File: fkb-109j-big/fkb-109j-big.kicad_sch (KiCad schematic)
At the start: 187 parts

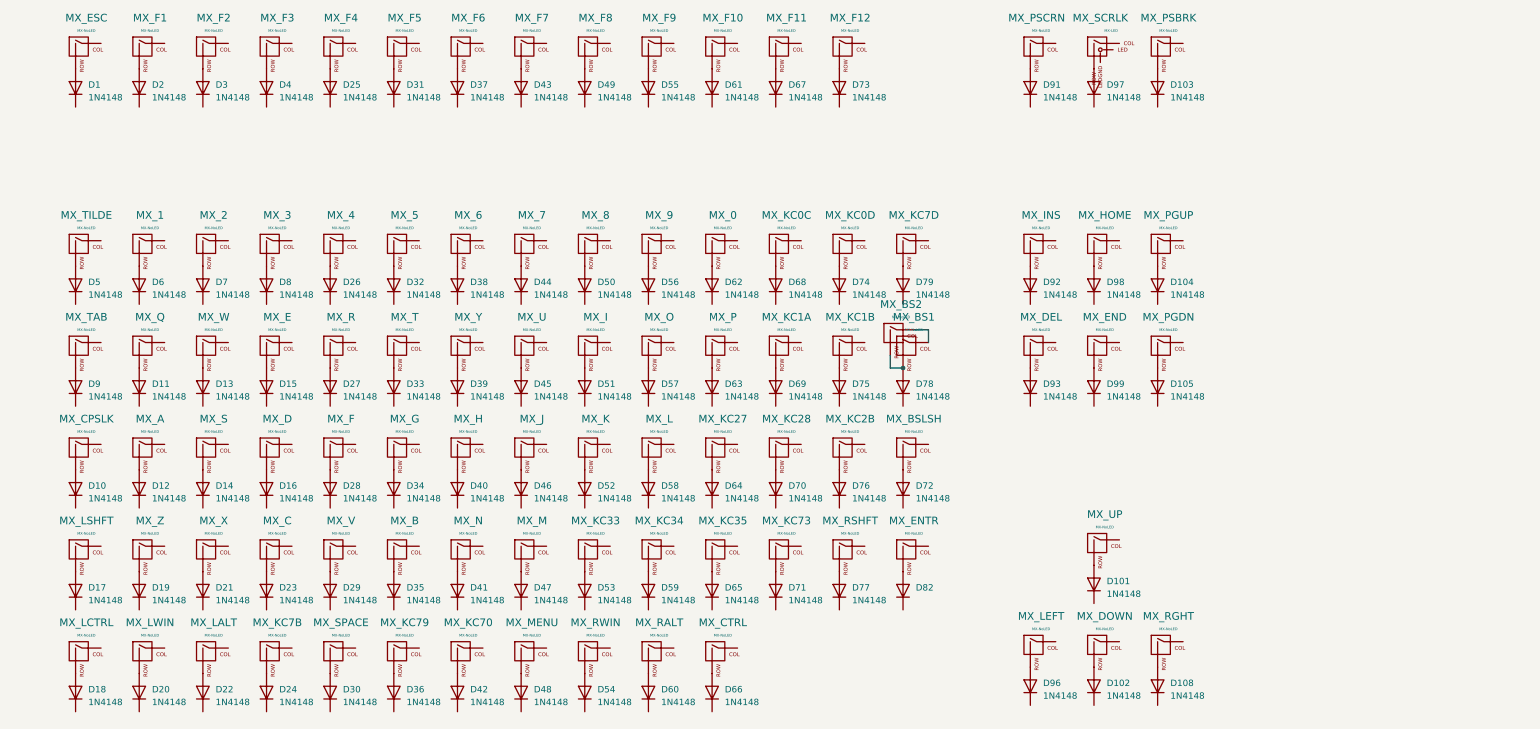
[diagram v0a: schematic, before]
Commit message: start board layout
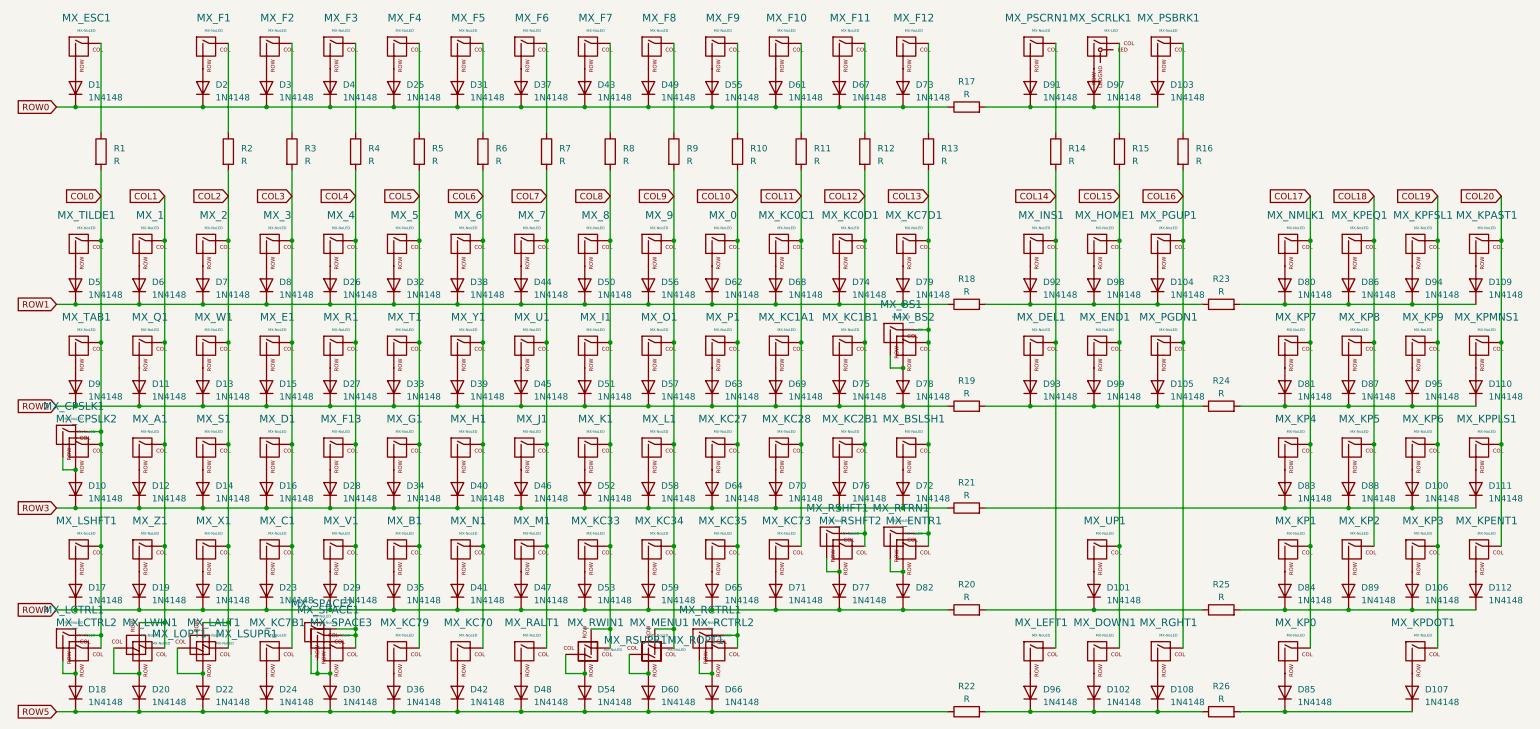
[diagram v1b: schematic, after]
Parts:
- added D100, D106, D107, D109, D110, D111, D112, D80, D81, D83, D84, D85, D86, D87, D88, D89, D94, D95: 1N4148, Diode_THT:D_DO-35_SOD27_P7.62mm_Horizontal, symbol Diode:1N4148
- added MX_CPSLK1, MX_LSUPR1, MX_RSUPR1: MX-NoLED, Alps_Only:ALPS-1.5U, symbol MX_Alps_Hybrid:MX-NoLED
- added MX_KP0, MX_KP1, MX_KP2, MX_KP3, MX_KP4, MX_KP5, MX_KP6, MX_KP7, MX_KP8, MX_KP9, MX_KPAST1, MX_KPDOT1, MX_KPEQ1, MX_KPFSL1, MX_KPMNS1, MX_KPPLS1, MX_NMLK1: MX-NoLED, Alps_Only:ALPS-1U, symbol MX_Alps_Hybrid:MX-NoLED
- added MX_KPENT1: MX-NoLED, Alps_Only:ALPS-2U, symbol MX_Alps_Hybrid:MX-NoLED
- added MX_LCTRL1, MX_LOPT1, MX_RCTRL1, MX_ROPT1: MX-NoLED, Alps_Only:ALPS-1.25U, symbol MX_Alps_Hybrid:MX-NoLED
- added MX_RSHFT1: MX-NoLED, Alps_Only:ALPS-2.75U, symbol MX_Alps_Hybrid:MX-NoLED
- added MX_RTRN1: MX-NoLED, Alps_Only:ALPS-2.25U, symbol MX_Alps_Hybrid:MX-NoLED
- added MX_SPACE1: MX-NoLED, Alps_Only:ALPS-6.5U, symbol MX_Alps_Hybrid:MX-NoLED
- added MX_SPACE2: MX-NoLED, Alps_Only:ALPS-6.25U, symbol MX_Alps_Hybrid:MX-NoLED
- added R1, R10, R11, R12, R13, R14, R15, R16, R17, R18, R19, R2, R20, R21, R22, R23, R24, R25, R26, R3, R4, R5, R6, R7, R8, R9: R, Resistor_THT:R_Axial_DIN0207_L6.3mm_D2.5mm_P10.16mm_Horizontal, symbol Device:R
- MX_0, MX_1, MX_2, MX_3, MX_4, MX_5, MX_6, MX_7, MX_8, MX_9, MX_F1, MX_F10, MX_F11, MX_F12, MX_F2, MX_F3, MX_F4, MX_F5, MX_F6, MX_F7, MX_F8, MX_F9, MX_KC27, MX_KC28, MX_KC33, MX_KC34, MX_KC35, MX_KC73: footprint (none) -> Alps_Only:ALPS-1U
- MX_A1: renamed from MX_A; footprint (none) -> Alps_Only:ALPS-1U
- MX_B1: renamed from MX_B; footprint (none) -> Alps_Only:ALPS-1U
- MX_BS2: renamed from MX_BS1; footprint Alps_Only:ALPS-1U -> Alps_Only:ALPS-2U
- MX_BSLSH1: renamed from MX_BSLSH; footprint (none) -> Alps_Only:ALPS-1.5U
- MX_C1: renamed from MX_C; footprint (none) -> Alps_Only:ALPS-1U
- MX_CPSLK2: renamed from MX_CPSLK; footprint (none) -> Alps_Only:ALPS-1.75U
- MX_D1: renamed from MX_D; footprint (none) -> Alps_Only:ALPS-1U
- MX_DEL1: renamed from MX_DEL; footprint (none) -> Alps_Only:ALPS-1U
- MX_DOWN1: renamed from MX_DOWN; footprint (none) -> Alps_Only:ALPS-1U
- MX_E1: renamed from MX_E; footprint (none) -> Alps_Only:ALPS-1U
- MX_END1: renamed from MX_END; footprint (none) -> Alps_Only:ALPS-1U
- MX_ENTR1: renamed from MX_ENTR; footprint (none) -> Alps_Only:ALPS-2U
- MX_ESC1: renamed from MX_ESC; footprint (none) -> Alps_Only:ALPS-1U
- MX_F13: renamed from MX_F; footprint (none) -> Alps_Only:ALPS-1U
- MX_G1: renamed from MX_G; footprint (none) -> Alps_Only:ALPS-1U
- MX_H1: renamed from MX_H; footprint (none) -> Alps_Only:ALPS-1U
- MX_HOME1: renamed from MX_HOME; footprint (none) -> Alps_Only:ALPS-1U
- MX_I1: renamed from MX_I; footprint (none) -> Alps_Only:ALPS-1U
- MX_INS1: renamed from MX_INS; footprint (none) -> Alps_Only:ALPS-1U
- MX_J1: renamed from MX_J; footprint (none) -> Alps_Only:ALPS-1U
- MX_K1: renamed from MX_K; footprint (none) -> Alps_Only:ALPS-1U
- MX_KC0C1: renamed from MX_KC0C; footprint (none) -> Alps_Only:ALPS-1U
- MX_KC0D1: renamed from MX_KC0D; footprint (none) -> Alps_Only:ALPS-1U
- MX_KC1A1: renamed from MX_KC1A; footprint (none) -> Alps_Only:ALPS-1U
- MX_KC1B1: renamed from MX_KC1B; footprint (none) -> Alps_Only:ALPS-1U
- MX_KC2B1: renamed from MX_KC2B; footprint (none) -> Alps_Only:ALPS-1U
- MX_KC70, MX_KC79: footprint (none) -> Alps_Only:ALPS-1.25U
- MX_KC7B1: renamed from MX_KC7B; footprint (none) -> Alps_Only:ALPS-1.25U
- MX_KC7D1: renamed from MX_KC7D; footprint (none) -> Alps_Only:ALPS-1U
- MX_L1: renamed from MX_L; footprint (none) -> Alps_Only:ALPS-1U
- MX_LALT1: renamed from MX_LALT; footprint (none) -> Alps_Only:ALPS-1.25U
- MX_LCTRL2: renamed from MX_LCTRL; footprint (none) -> Alps_Only:ALPS-1.5U
- MX_LEFT1: renamed from MX_LEFT; footprint (none) -> Alps_Only:ALPS-1U
- MX_LSHFT1: renamed from MX_LSHFT; footprint (none) -> Alps_Only:ALPS-2.25U
- MX_LWIN1: renamed from MX_LWIN; footprint (none) -> Alps_Only:ALPS-1.25U
- MX_M1: renamed from MX_M; footprint (none) -> Alps_Only:ALPS-1U
- MX_MENU1: renamed from MX_MENU; footprint (none) -> Alps_Only:ALPS-1.25U
- MX_N1: renamed from MX_N; footprint (none) -> Alps_Only:ALPS-1U
- MX_O1: renamed from MX_O; footprint (none) -> Alps_Only:ALPS-1U
- MX_P1: renamed from MX_P; footprint (none) -> Alps_Only:ALPS-1U
- MX_PGDN1: renamed from MX_PGDN; footprint (none) -> Alps_Only:ALPS-1U
- MX_PGUP1: renamed from MX_PGUP; footprint (none) -> Alps_Only:ALPS-1U
- MX_PSBRK1: renamed from MX_PSBRK; footprint (none) -> Alps_Only:ALPS-1U
- MX_PSCRN1: renamed from MX_PSCRN; footprint (none) -> Alps_Only:ALPS-1U
- MX_Q1: renamed from MX_Q; footprint (none) -> Alps_Only:ALPS-1U
- MX_R1: renamed from MX_R; footprint (none) -> Alps_Only:ALPS-1U
- MX_RALT1: renamed from MX_RALT; footprint (none) -> Alps_Only:ALPS-1.25U
- MX_RCTRL2: renamed from MX_CTRL; footprint (none) -> Alps_Only:ALPS-1.5U
- MX_RGHT1: renamed from MX_RGHT; footprint (none) -> Alps_Only:ALPS-1U
- MX_RSHFT2: renamed from MX_RSHFT; footprint (none) -> Alps_Only:ALPS-1.75U
- MX_RWIN1: renamed from MX_RWIN; footprint (none) -> Alps_Only:ALPS-1.25U
- MX_S1: renamed from MX_S; footprint (none) -> Alps_Only:ALPS-1U
- MX_SCRLK1: renamed from MX_SCRLK; footprint (none) -> Alps_Only:ALPS-1U
- MX_SPACE3: renamed from MX_SPACE; footprint (none) -> Alps_Only:ALPS-2.5U
- MX_T1: renamed from MX_T; footprint (none) -> Alps_Only:ALPS-1U
- MX_TAB1: renamed from MX_TAB; footprint (none) -> Alps_Only:ALPS-1.5U
- MX_TILDE1: renamed from MX_TILDE; footprint (none) -> Alps_Only:ALPS-1U
- MX_U1: renamed from MX_U; footprint (none) -> Alps_Only:ALPS-1U
- MX_UP1: renamed from MX_UP; footprint (none) -> Alps_Only:ALPS-1U
- MX_V1: renamed from MX_V; footprint (none) -> Alps_Only:ALPS-1U
- MX_W1: renamed from MX_W; footprint (none) -> Alps_Only:ALPS-1U
- MX_X1: renamed from MX_X; footprint (none) -> Alps_Only:ALPS-1U
- MX_Y1: renamed from MX_Y; footprint (none) -> Alps_Only:ALPS-1U
- MX_Z1: renamed from MX_Z; footprint (none) -> Alps_Only:ALPS-1U
- renumbered MX_BS2 to MX_BS1
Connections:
- net COL2: now reaches MX_S1.1 (COL)
- net COL2: now also MX_2.1 (COL), MX_LALT1.1 (COL), MX_W1.1 (COL), MX_X1.1 (COL), MX_LSUPR1.2 (ROW), R2.2
- net at D97.1 (K): now also D103.1 (K), D91.1 (K), R17.2
- net ROW4: now reaches D53.1 (K)
- net ROW4: now also D17.1 (K), D19.1 (K), D21.1 (K), D23.1 (K), D29.1 (K), D35.1 (K), D41.1 (K), D47.1 (K), D59.1 (K), D65.1 (K), D71.1 (K), D77.1 (K), D82.1 (K), R20.1
- net COL9: now reaches MX_O1.1 (COL)
- net COL9: now also MX_9.1 (COL), MX_KC34.1 (COL), MX_L1.1 (COL), MX_MENU1.1 (COL), MX_ROPT1.2 (ROW), R9.2
- net ROW5: now reaches D24.1 (K)
- net ROW5: now also D18.1 (K), D20.1 (K), D22.1 (K), D30.1 (K), D36.1 (K), D42.1 (K), D48.1 (K), D54.1 (K), D60.1 (K), D66.1 (K), R22.1
- net ROW3: now reaches D34.1 (K)
- net ROW3: now also D10.1 (K), D12.1 (K), D14.1 (K), D16.1 (K), D28.1 (K), D40.1 (K), D46.1 (K), D52.1 (K), D58.1 (K), D64.1 (K), D70.1 (K), D72.1 (K), D76.1 (K), R21.1
- net COL13: now reaches MX_BS1.1 (COL), MX_BS2.1 (COL)
- net COL13: now also MX_BSLSH1.1 (COL), MX_ENTR1.1 (COL), MX_KC7D1.1 (COL), MX_RTRN1.1 (COL), R13.2
- net ROW1: now reaches D68.1 (K)
- net ROW1: now also D26.1 (K), D32.1 (K), D38.1 (K), D44.1 (K), D5.1 (K), D50.1 (K), D56.1 (K), D6.1 (K), D62.1 (K), D7.1 (K), D74.1 (K), D79.1 (K), D8.1 (K), R18.1
- net COL10: now reaches MX_P1.1 (COL)
- net COL10: now also MX_0.1 (COL), MX_KC27.1 (COL), MX_KC35.1 (COL), MX_RCTRL2.1 (COL), MX_RCTRL1.1 (COL), R10.2
- net ROW0: now reaches D3.1 (K)
- net ROW0: now also D1.1 (K), D2.1 (K), D25.1 (K), D31.1 (K), D37.1 (K), D4.1 (K), D43.1 (K), D49.1 (K), D55.1 (K), D61.1 (K), D67.1 (K), D73.1 (K), R17.1
- net COL11: now reaches MX_KC73.1 (COL)
- net COL11: now also MX_KC0C1.1 (COL), MX_KC1A1.1 (COL), MX_KC28.1 (COL), R11.2
- net at MX_F6.1 (COL): now also R7.1
- net ROW2: now reaches D13.1 (K)
- net ROW2: now also D11.1 (K), D15.1 (K), D27.1 (K), D33.1 (K), D39.1 (K), D45.1 (K), D51.1 (K), D57.1 (K), D63.1 (K), D69.1 (K), D75.1 (K), D78.1 (K), D9.1 (K), R19.1
- net COL7: now reaches MX_U1.1 (COL)
- net COL7: now also MX_7.1 (COL), MX_J1.1 (COL), MX_M1.1 (COL), MX_RALT1.1 (COL), R7.2
- net at D96.1 (K): now also D102.1 (K), D108.1 (K), R22.2, R26.1
- net COL4: now reaches MX_V1.1 (COL)
- net COL4: now also MX_4.1 (COL), MX_F13.1 (COL), MX_R1.1 (COL), MX_SPACE3.1 (COL), MX_SPACE1.1 (COL), MX_SPACE2.1 (COL), R4.2
- net at D20.2 (A), MX_LWIN1.2 (ROW): now also MX_LOPT1.1 (COL)
- net COL1: now reaches MX_LWIN1.1 (COL)
- net COL1: now also MX_1.1 (COL), MX_A1.1 (COL), MX_Q1.1 (COL), MX_Z1.1 (COL), MX_LOPT1.2 (ROW)
- net COL6: now reaches MX_H1.1 (COL)
- net COL6: now also MX_6.1 (COL), MX_KC70.1 (COL), MX_N1.1 (COL), MX_Y1.1 (COL), R6.2
- net at D30.2 (A), MX_SPACE3.2 (ROW): now also MX_SPACE1.2 (ROW), MX_SPACE2.2 (ROW)
- net COL0: now reaches MX_TAB1.1 (COL)
- net COL0: now also MX_CPSLK2.1 (COL), MX_LCTRL2.1 (COL), MX_LSHFT1.1 (COL), MX_TILDE1.1 (COL), MX_CPSLK1.1 (COL), MX_LCTRL1.1 (COL), R1.2
- net at D93.1 (K): now also D105.1 (K), D99.1 (K), R19.2, R24.1
- net COL8: now reaches MX_I1.1 (COL)
- net COL8: now also MX_8.1 (COL), MX_K1.1 (COL), MX_KC33.1 (COL), MX_RWIN1.1 (COL), MX_RSUPR1.2 (ROW), R8.2
- net at D82.2 (A), MX_ENTR1.2 (ROW): now also MX_RTRN1.2 (ROW)
- net COL5: now reaches MX_5.1 (COL)
- net COL5: now also MX_B1.1 (COL), MX_G1.1 (COL), MX_KC79.1 (COL), MX_T1.1 (COL), R5.2
- net COL12: now reaches MX_KC0D1.1 (COL)
- net COL12: now also MX_KC1B1.1 (COL), MX_KC2B1.1 (COL), MX_RSHFT2.1 (COL), MX_RSHFT1.1 (COL), R12.2
- net at MX_MENU1.2 (ROW): now also D60.2 (A), MX_ROPT1.1 (COL); no longer D48.2 (A)
- net at D77.2 (A), MX_RSHFT2.2 (ROW): now also MX_RSHFT1.2 (ROW)
- net at D22.2 (A), MX_LALT1.2 (ROW): now also MX_LSUPR1.1 (COL)
- net at MX_PSCRN1.1 (COL): now also R14.1
- net at D54.2 (A), MX_RWIN1.2 (ROW): now also MX_RSUPR1.1 (COL)
- net at MX_F12.1 (COL): now also R13.1
- net at MX_F5.1 (COL): now also R6.1
- net COL14: now reaches MX_DEL1.1 (COL)
- net COL14: now also MX_INS1.1 (COL), MX_LEFT1.1 (COL), R14.2
- net at MX_F10.1 (COL): now also R11.1
- net at D98.1 (K): now also D104.1 (K), D92.1 (K), R18.2, R23.1
- net at MX_F4.1 (COL): now also R5.1
- net at D18.2 (A), MX_LCTRL2.2 (ROW): now also MX_LCTRL1.2 (ROW)
- net at MX_F8.1 (COL): now also R9.1
- net at MX_ESC1.1 (COL): now also R1.1
- net at MX_F7.1 (COL): now also R8.1
- net COL16: now reaches MX_PGDN1.1 (COL)
- net COL16: now also MX_PGUP1.1 (COL), MX_RGHT1.1 (COL), R16.2
- net at D66.2 (A), MX_RCTRL2.2 (ROW): now also MX_RCTRL1.2 (ROW)
- net at MX_F9.1 (COL): now also R10.1
- net at MX_RALT1.2 (ROW): now also D48.2 (A); no longer D60.2 (A)
- net COL15: now reaches MX_HOME1.1 (COL)
- net COL15: now also MX_DOWN1.1 (COL), MX_END1.1 (COL), MX_UP1.1 (COL), R15.2
- net at D101.1 (K): now also R20.2, R25.1
- net at MX_SCRLK1.1 (COL): now also R15.1
- net COL3: now reaches MX_KC7B1.1 (COL)
- net COL3: now also MX_3.1 (COL), MX_C1.1 (COL), MX_D1.1 (COL), MX_E1.1 (COL), R3.2
- net at MX_F1.1 (COL): now also R2.1
- net at MX_F3.1 (COL): now also R4.1
- net at MX_F11.1 (COL): now also R12.1
- net at D10.2 (A), MX_CPSLK2.2 (ROW): now also MX_CPSLK1.2 (ROW)
- net at MX_F2.1 (COL): now also R3.1
- net at MX_PSBRK1.1 (COL): now also R16.1
- new net: D100.1 (K), D111.1 (K), D83.1 (K), D88.1 (K), R21.2
- new net: D106.1 (K), D112.1 (K), D84.1 (K), D89.1 (K), R25.2
- new net: D84.2 (A), MX_KP1.2 (ROW)
- new net: D81.2 (A), MX_KP7.2 (ROW)
- new net: D109.1 (K), D80.1 (K), D86.1 (K), D94.1 (K), R23.2
- new net: D89.2 (A), MX_KP2.2 (ROW)
- new net: D107.2 (A), MX_KPDOT1.2 (ROW)
- new net: D80.2 (A), MX_NMLK1.2 (ROW)
- new net: D107.1 (K), D85.1 (K), R26.2
- new net: D85.2 (A), MX_KP0.2 (ROW)
- new net: D110.1 (K), D81.1 (K), D87.1 (K), D95.1 (K), R24.2
- new net: D110.2 (A), MX_KPMNS1.2 (ROW)
- new net: D112.2 (A), MX_KPENT1.2 (ROW)
- new net: D86.2 (A), MX_KPEQ1.2 (ROW)
- new net: D88.2 (A), MX_KP5.2 (ROW)
- new net: D111.2 (A), MX_KPPLS1.2 (ROW)
- new net: D83.2 (A), MX_KP4.2 (ROW)
- new net: D95.2 (A), MX_KP9.2 (ROW)
- new net: D100.2 (A), MX_KP6.2 (ROW)
- new net: D94.2 (A), MX_KPFSL1.2 (ROW)
- new net: D87.2 (A), MX_KP8.2 (ROW)
- new net: D109.2 (A), MX_KPAST1.2 (ROW)
- new net: D106.2 (A), MX_KP3.2 (ROW)
- new net COL17: MX_KP0.1 (COL), MX_KP1.1 (COL), MX_KP4.1 (COL), MX_KP7.1 (COL), MX_NMLK1.1 (COL)
- new net COL18: MX_KP2.1 (COL), MX_KP5.1 (COL), MX_KP8.1 (COL), MX_KPEQ1.1 (COL)
- new net COL19: MX_KP3.1 (COL), MX_KP6.1 (COL), MX_KP9.1 (COL), MX_KPDOT1.1 (COL), MX_KPFSL1.1 (COL)
- new net COL20: MX_KPAST1.1 (COL), MX_KPENT1.1 (COL), MX_KPMNS1.1 (COL), MX_KPPLS1.1 (COL)
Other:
- moved on the sheet: D101, D102, D108, D2, D25, D3, D31, D37, D4, D43, D49, D55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

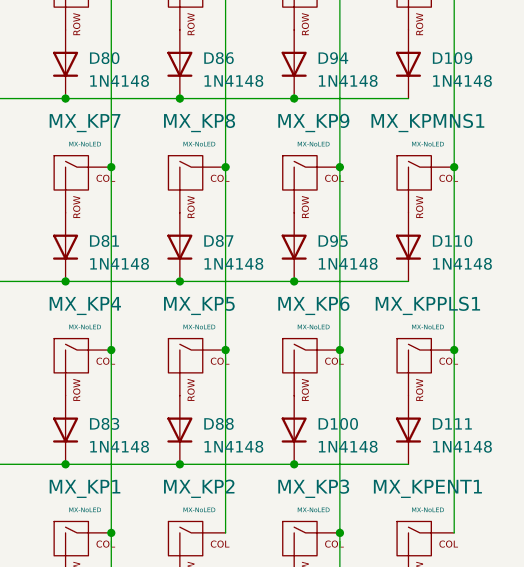
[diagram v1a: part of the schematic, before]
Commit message: continue layout
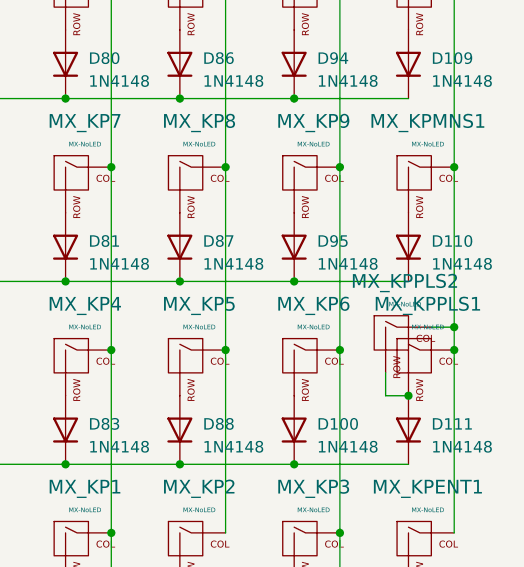
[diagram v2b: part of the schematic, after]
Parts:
- added MX_KPPLS2: MX-NoLED, Alps_Only:ALPS-2U, symbol MX_Alps_Hybrid:MX-NoLED
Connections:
- net COL20: now also MX_KPPLS2.1 (COL)
- net at D111.2 (A), MX_KPPLS1.2 (ROW): now also MX_KPPLS2.2 (ROW)
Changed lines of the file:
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@@
   (junction (at 86.36 138.43) (diameter 0) (color 0 0 0 0)
   )
+  (junction (at 307.34 102.87) (diameter 0) (color 0 0 0 0)
+  )
   (junction (at 193.04 105.41) (diameter 0) (color 0 0 0 0)
   )
@@
   (junction (at 40.64 125.73) (diameter 0) (color 0 0 0 0)
   )
+  (junction (at 302.26 110.49) (diameter 0) (color 0 0 0 0)
+  )
   (junction (at 231.14 85.09) (diameter 0) (color 0 0 0 0)
   )
@@
     (stroke (width 0) (type default))
   )
-  (wire (pts (xy 307.34 85.09) (xy 307.34 105.41))
+  (wire (pts (xy 307.34 85.09) (xy 307.34 102.87))
     (stroke (width 0) (type default))
   )
@@
     (stroke (width 0) (type default))
   )
+  (wire (pts (xy 299.72 107.95) (xy 299.72 110.49))
+    (stroke (width 0) (type default))
+  )
   (wire (pts (xy 25.4 102.87) (xy 27.94 102.87))
     (stroke (width 0) (type default))
@@
     (stroke (width 0) (type default))
   )
+  (wire (pts (xy 304.8 102.87) (xy 307.34 102.87))
+    (stroke (width 0) (type default))
+  )
   (wire (pts (xy 40.64 140.97) (xy 40.64 146.05))
     (stroke (width 0) (type default))
@@
     (stroke (width 0) (type default))
   )
+  (wire (pts (xy 299.72 110.49) (xy 302.26 110.49))
+    (stroke (width 0) (type default))
+  )
   (wire (pts (xy 66.04 25.4) (xy 66.04 43.18))
     (stroke (width 0) (type default))
@@
     (stroke (width 0) (type default))
   )
+  (wire (pts (xy 307.34 102.87) (xy 307.34 105.41))
+    (stroke (width 0) (type default))
+  )
   (wire (pts (xy 116.84 50.8) (xy 116.84 64.77))
     (stroke (width 0) (type default))
@@
         )
       )
+    )
+  )
+  (symbol (lib_id "MX_Alps_Hybrid:MX-NoLED") (at 300.99 104.14 0) (unit 1)
+    (in_bom yes) (on_board yes) (dnp no) (fields_autoplaced)
+    (property "Reference" "MX_KPPLS2" (at 301.8732 97.79 0)
+      (effects (font (size 1.524 1.524)))
+    )
+    (property "Value" "MX-NoLED" (at 301.8732 100.33 0)
+      (effects (font (size 0.508 0.508)))
+    )
+    (property "Footprint" "Alps_Only:ALPS-2U" (at 285.115 104.775 0)
+      (effects (font (size 1.524 1.524)) hide)
+    )
+    (property "Datasheet" "" (at 285.115 104.775 0)
+      (effects (font (size 1.524 1.524)) hide)
+    )
+    (pin "1")
+    (pin "2")
+    (instances
+      (project "fkb-109j-big"
+        (path "/b3d18fbb-85f6-4085-bc49-223707581c3b"
+          (reference "MX_KPPLS2") (unit 1)
+        )
+      )
